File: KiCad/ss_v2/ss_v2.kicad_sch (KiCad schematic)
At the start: 59 parts, among them J1 PJ-313D-B-SMT, J2 UJC-HP-M-G-5-MSMT-TR, J3 DC-005-20A, J4 Conn_02x03_Top_Bottom, J5 Conn_02x03_Counter_Clockwise, J6 Conn_01x08_Pin, J7 Conn_01x04, Q1 BSN20, Q2 IRF7416TRPBF, Q3 BSN20, SW1 TS-1093C-A15, SW2 TS-1093C-A15, SW3 TS-1093C-A15, SW4 TS-1093C-A15, U1 ATMEGA328P-AU, U2 LM321, U3 TPS62125DSG, U4 FUSB302B10MPX, Y1 Crystal

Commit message: korrektur der Fehlenden Footprints
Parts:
- J4: footprint (none) -> Connector_IDC:IDC-Header_2x03_P2.54mm_Vertical
- R27: footprint (none) -> Resistor_SMD:R_1206_3216Metric_Pad1.30x1.75mm_HandSolder
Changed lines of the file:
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@@
       (effects (font (size 1.27 1.27)))
     )
-    (property "Footprint" "" (at 43.815 25.4 0)
+    (property "Footprint" "Connector_IDC:IDC-Header_2x03_P2.54mm_Vertical" (at 43.815 25.4 0)
       (effects (font (size 1.27 1.27)) hide)
     )
@@
       (effects (font (size 1.27 1.27)) (justify left))
     )
-    (property "Footprint" "" (at 212.852 75.565 90)
-      (effects (font (size 1.27 1.27)) hide)
-    )
+    (property "Footprint" "Resistor_SMD:R_1206_3216Metric_Pad1.30x1.75mm_HandSolder" (at 212.852 75.565 90)
+      (effects (font (size 1.27 1.27)) hide)
+    )

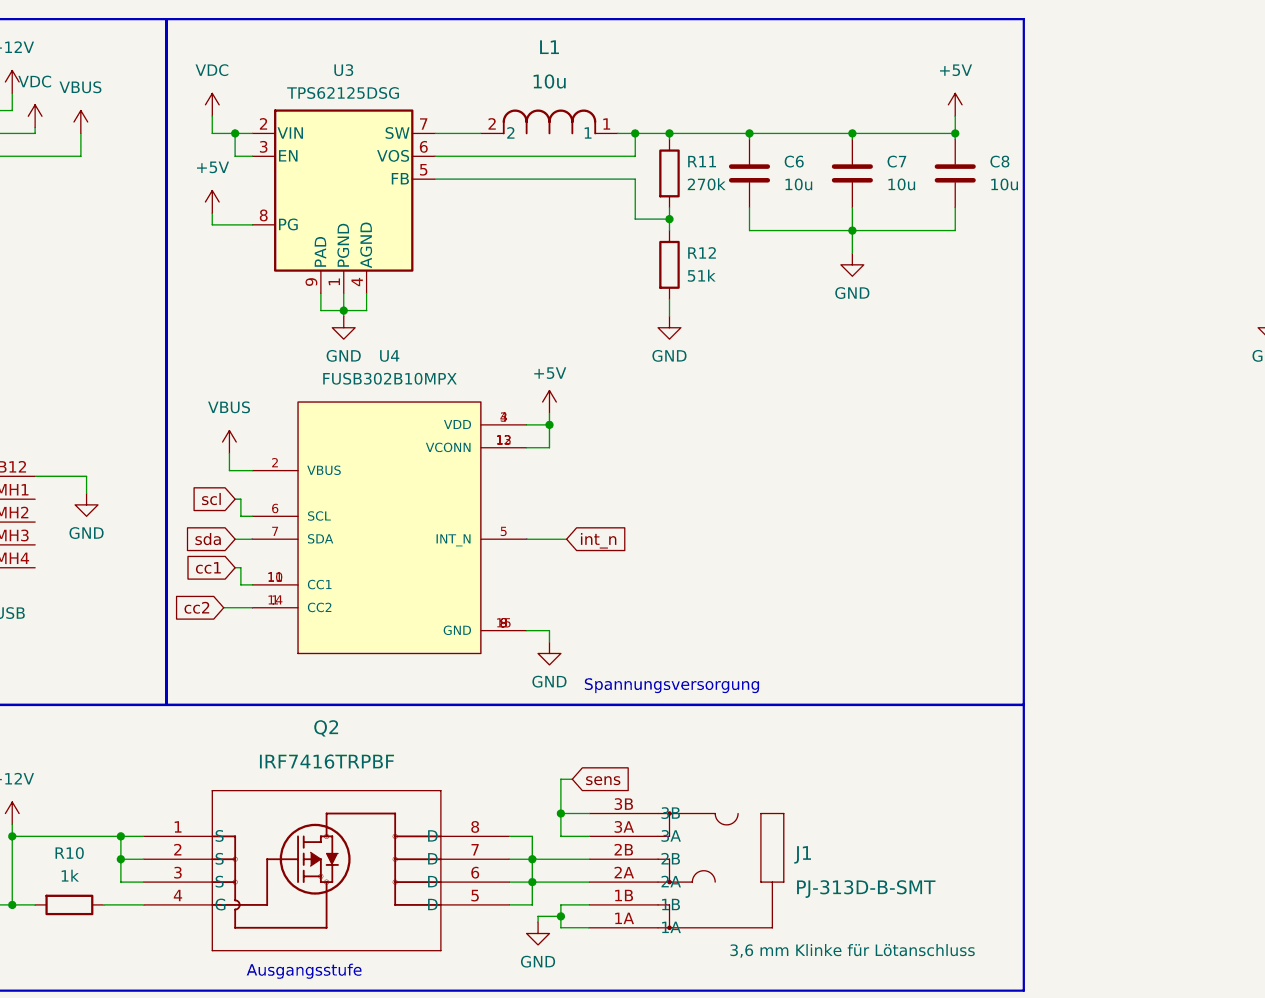
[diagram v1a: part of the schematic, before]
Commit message: Erster Routing Versuch
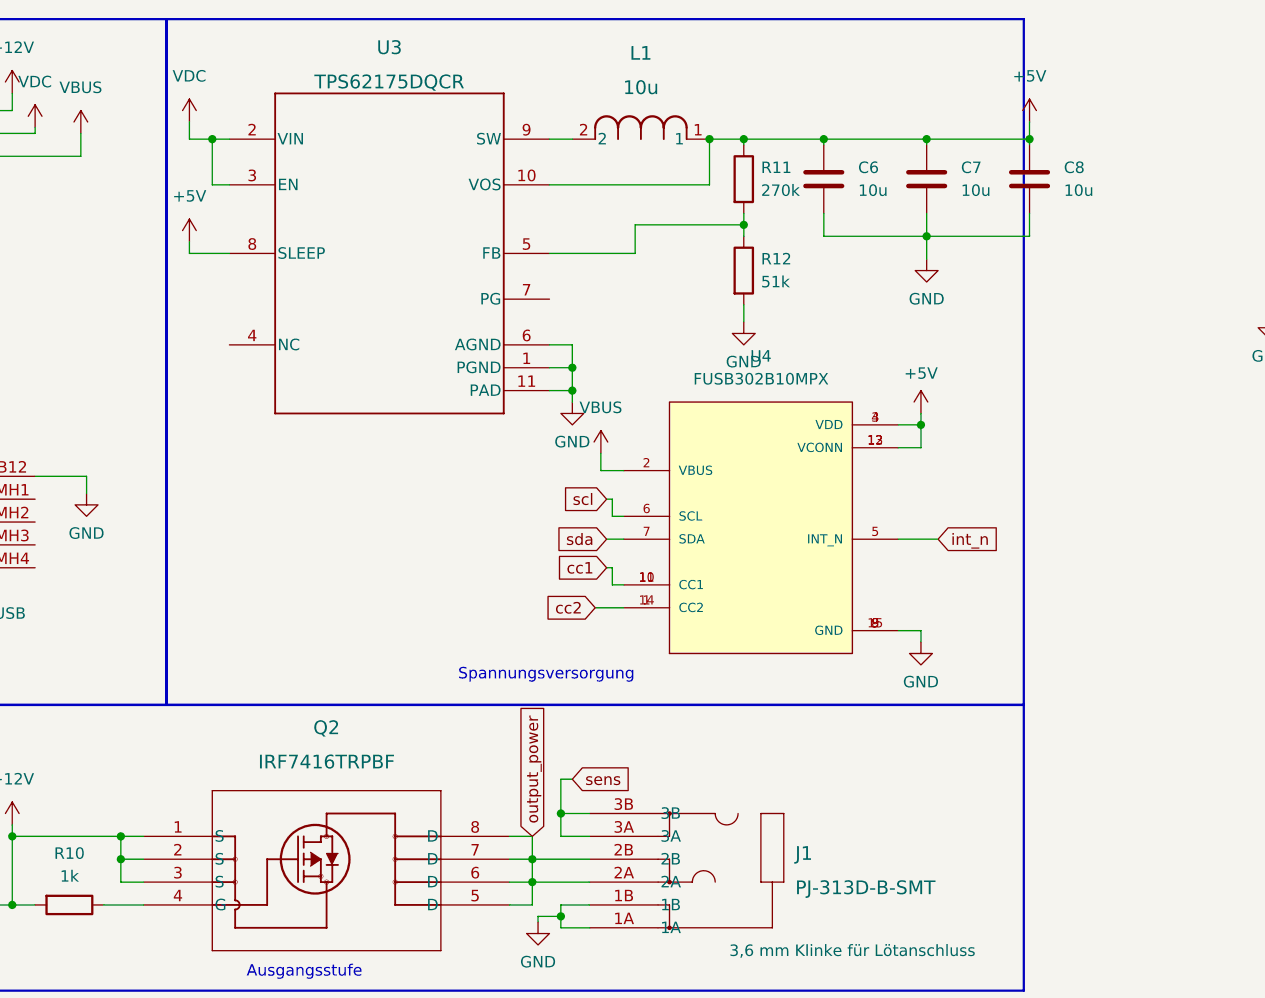
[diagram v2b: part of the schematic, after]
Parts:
- removed U3: TPS62125DSG, Package_SON:WSON-8-1EP_2x2mm_P0.5mm_EP0.9x1.6mm_ThermalVias, symbol Regulator_Switching:TPS62125DSG
- added U3: TPS62175DQCR, DQC0010A, symbol TPS62175DQCR:TPS62175DQCR
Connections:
- net +5V: now also U3.10 (VOS), U3.8 (SLEEP)
- net GND: now also U3.1 (PGND), U3.11 (PAD), U3.6 (AGND)
- net VDC: now also U3.2 (VIN), U3.3 (EN)
- net at L1.2: now also U3.9 (SW)
- net at R11.2, R12.1: now also U3.5 (FB)
- net output_power: now reaches J1.2A, J1.2B, Q2.5 (D), Q2.6 (D), Q2.7 (D), Q2.8 (D)
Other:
- moved on the sheet: C6, C7, C8, L1, R11, R12, U4
